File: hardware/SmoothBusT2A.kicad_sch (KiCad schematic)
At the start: 13 parts, among them J1 Conn_ARM_SWD_TagConnect_TC203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, J2 BM03B-SRSS-TB_LF__SN_, J4 SM03B-SRSS-TB_LF__SN_, U1 ATTINY85-20SU, U2 MC7805BDTRKG

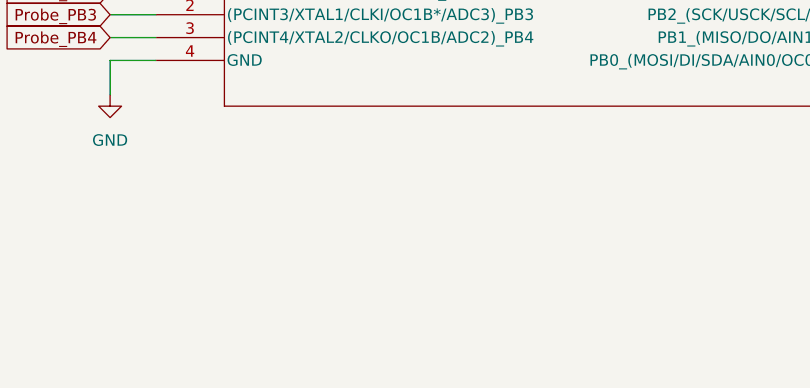
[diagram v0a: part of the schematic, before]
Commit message: version 1
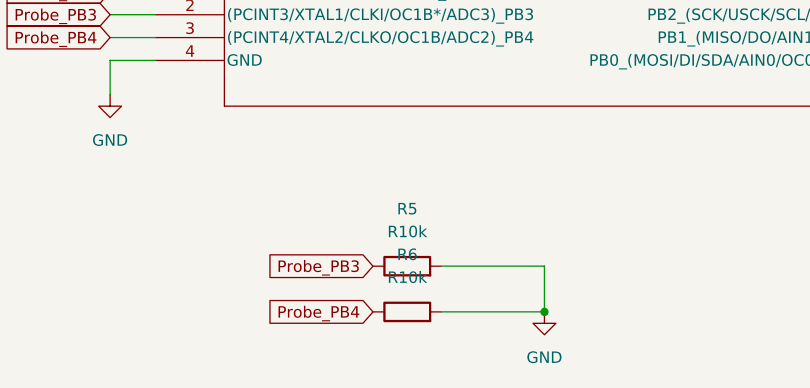
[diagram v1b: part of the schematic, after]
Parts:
- added R5, R6: R10k, Resistor_SMD:R_0201_0603Metric_Pad0.64x0.40mm_HandSolder, symbol Device:R
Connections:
- net GND: now also R5.2, R6.2
- net Probe_PB3: now also R5.1
- net Probe_PB4: now also R6.1
